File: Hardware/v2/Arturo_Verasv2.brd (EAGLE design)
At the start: 100 x 80 mm, 23 parts, among them T1 2SC1815, T3 2SC1815, T4 2SC1815, T5 2SC1815, T6 2SC1815, T7 2SC1815, T8 2SC1815, X1 22-23-2071

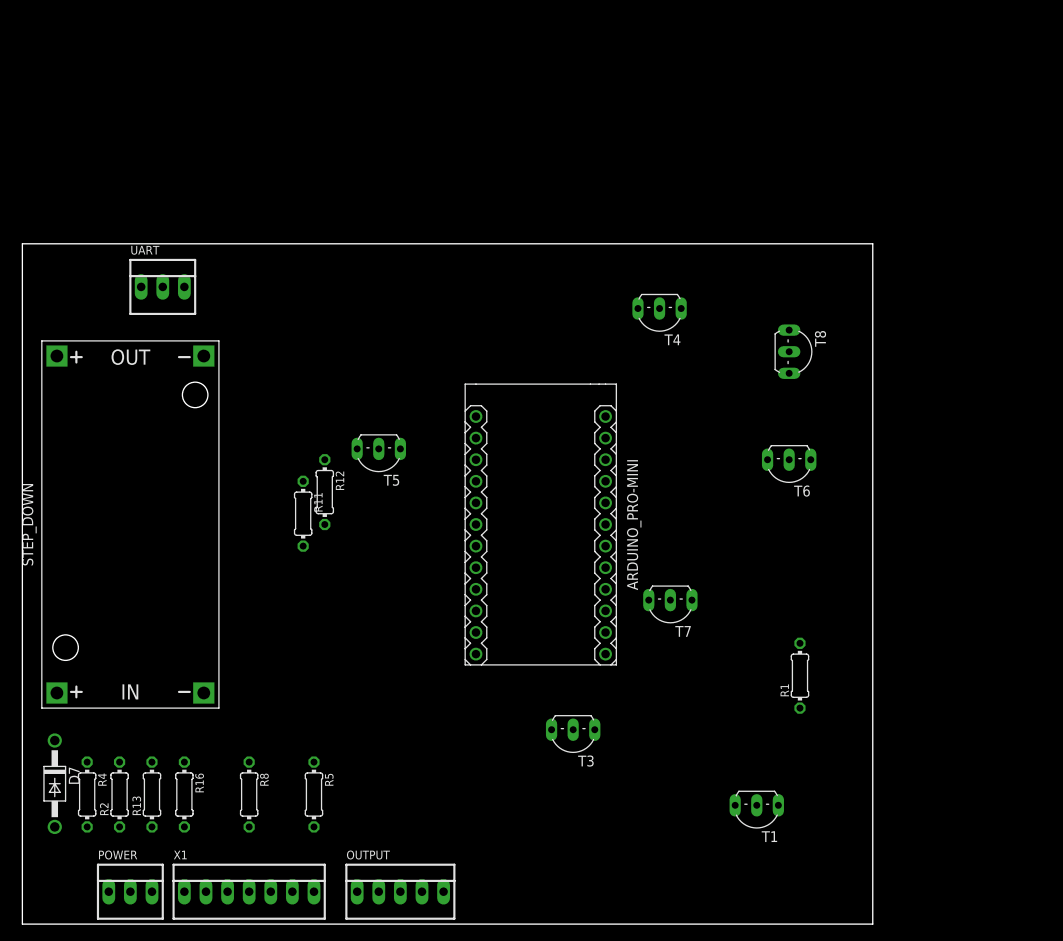
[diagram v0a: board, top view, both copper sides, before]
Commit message: Comentarios
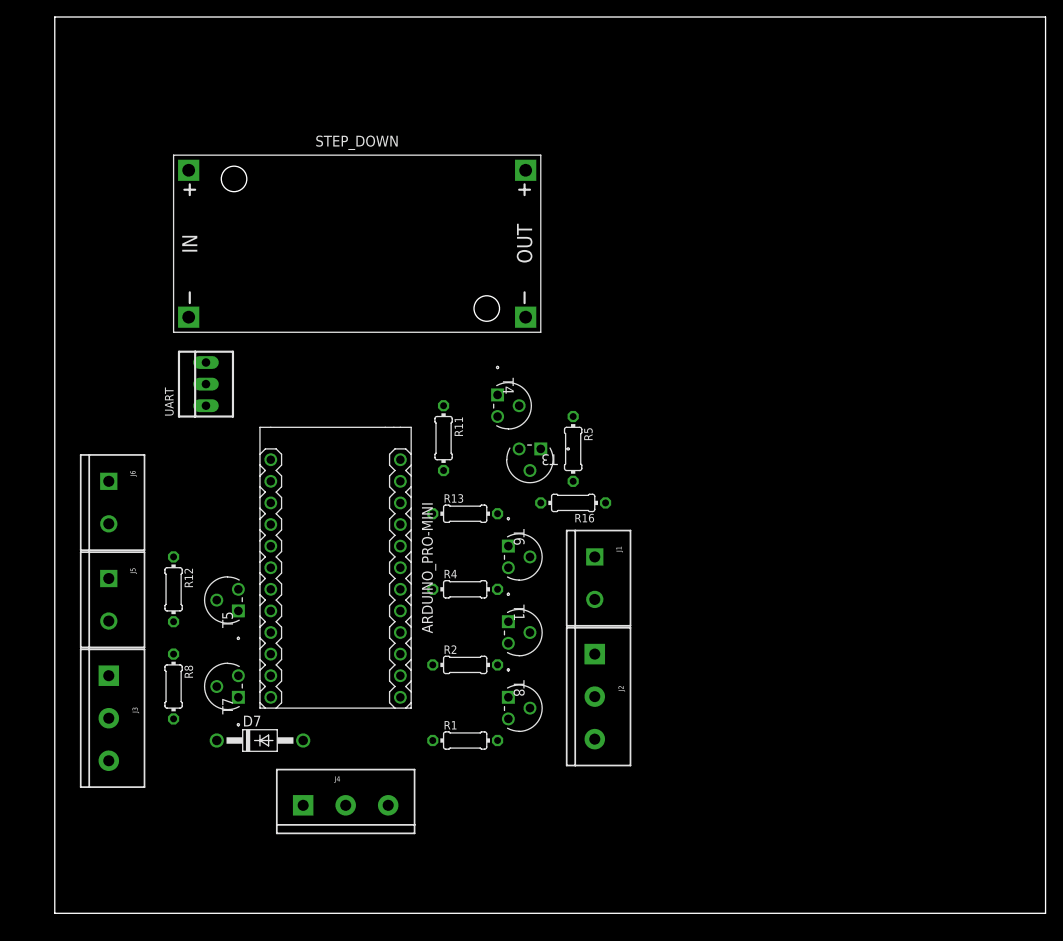
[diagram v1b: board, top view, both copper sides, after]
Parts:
- removed OUTPUT: 22-23-2051, con-molex:22-23-2051
- removed POWER: 22-23-2031, con-molex:22-23-2031
- removed X1: 22-23-2071, con-molex:22-23-2071
- added J1, J5, J6: (no value), SparkFun-Connectors:SCREWTERMINAL-5MM-2
- added J2, J3, J4: (no value), SparkFun-Connectors:SCREWTERMINAL-5MM-3
- T1, T3, T4, T5, T6, T7, T8: value 2SC1815 -> MPSA06; device transistor:TO92-ECB -> transistores:TO-92_2
- moved R16 57.1 mm to (64.8, 49.5), turned to 180 degrees
- moved T7 54.1 mm to (22.9, 29.2), turned to 90 degrees
- moved T8 52.9 mm to (59.7, 24.1)
- moved R5 50.8 mm to (64.8, 55.9)
- moved R4 50.6 mm to (52.1, 39.4), turned to 0 degrees
- moved R13 49.5 mm to (52.1, 48.3), turned to 0 degrees
- moved R2 43.4 mm to (52.1, 30.5), turned to 0 degrees
- moved STEP_DOWN 42.4 mm to (39.4, 80.0), turned to 0 degrees
- moved R1 40.1 mm to (52.1, 21.6), turned to 0 degrees
- moved T6 33.0 mm to (59.7, 41.9), turned to 270 degrees
- moved T1 32.8 mm to (59.7, 33.0), turned to 270 degrees
- moved T3 31.1 mm to (58.4, 53.3)
- moved T5 25.2 mm to (22.9, 39.4), turned to 90 degrees
- moved ARDUINO_PRO-MINI 24.7 mm to (36.8, 41.9)
- moved D7 24.7 mm to (27.9, 21.6), turned to 0 degrees
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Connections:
- net BUZZER_OUTPUT-: now also J1.2, T6.3; no longer OUTPUT.2, T6.C
- net CC_OUTPUT-: now also J2.2, T8.3; no longer OUTPUT.1, T8.C
- net DDOOR_INPUT-: now also J3.3; no longer X1.6
- net DENABLEDOOR_INPUT-: now also J3.1; no longer X1.5
- net DGENERAL_INPUT: now also T5.3; no longer T5.C
- net DIGNITION_INPUT: now also T7.3; no longer T7.C
- net DJAMMINGAUX_INPUT-: now also J6.2; no longer X1.4
- net DTDOUT1_INPUT-: now also J5.1; no longer X1.3
- net DTDOUT2_INPUT-: now also J6.1; no longer X1.1
- net GENERAL_INPUT+: now also J5.2; no longer X1.7
- net GND: now also J4.2, T1.1, T4.1, T5.1, T6.1, T7.1, T8.1; no longer POWER.2, T1.E, T4.E, T5.E, T6.E, T7.E, T8.E
- net IGNITION_INPUT+: now also J3.2; no longer X1.2
- net LED_OUTPUT-: now also J2.3; no longer OUTPUT.4
- net N$1: now also T5.2; no longer T5.B
- net N$2: now also T3.2; no longer T3.B
- net N$20: now also T4.2; no longer T4.B
- net N$22: now also T7.2; no longer T7.B
- net N$3: now also T8.2; no longer T8.B
- net N$4: now also T1.2; no longer T1.B
- net N$5: now also T6.2; no longer T6.B
- net N$6: now also T4.3; no longer T4.C
- net SPEAKER_OUTPUT-: now also J2.1, T1.3; no longer OUTPUT.3, T1.C
- net TDIN2_OUTPUT+: now also J1.1, T3.1; no longer OUTPUT.5, T3.E
- net VCC: no longer POWER.3
- net VIN: now also J4.1, T3.3; no longer POWER.1, T3.C
- net VOUT: now also J4.3
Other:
- board size 100 x 80 mm -> 116.5 x 105.4 mm
